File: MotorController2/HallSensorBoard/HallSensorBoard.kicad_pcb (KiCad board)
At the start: 2 copper layers, 13 x 23 mm, 6 parts, among them J1 Conn_01x07, J2 Conn_01x02, U1 S49E, U2 S49E, U3 S49E

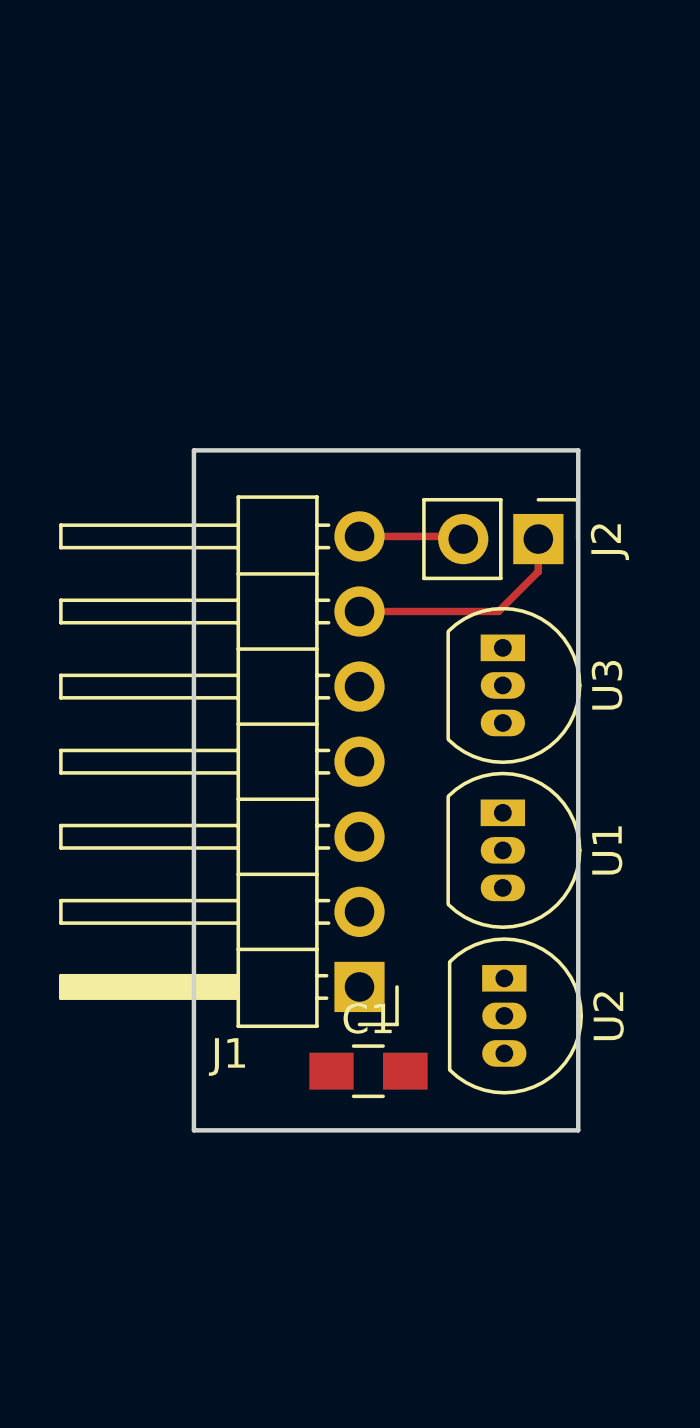
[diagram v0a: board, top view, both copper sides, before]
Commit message: Final board.
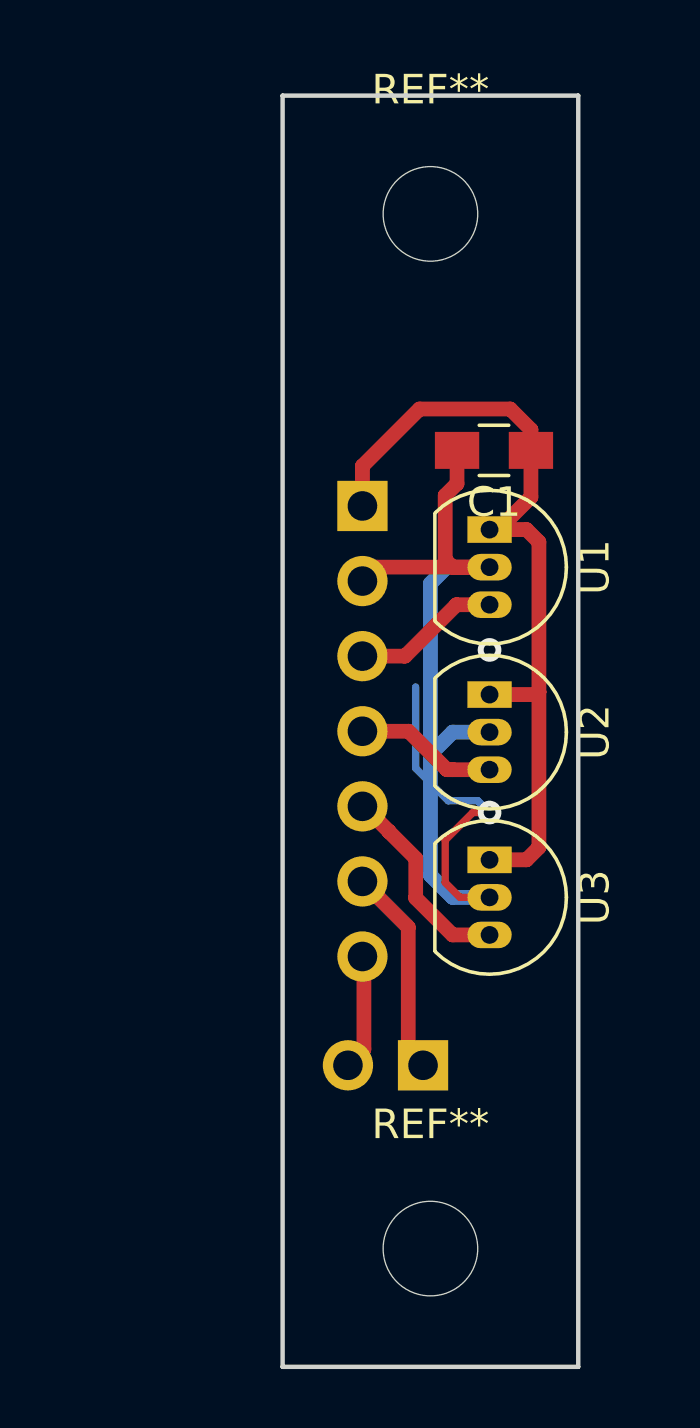
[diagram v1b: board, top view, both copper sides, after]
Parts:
- added REF**: MountingHole_3.2mm_M3, Mounting_Holes:MountingHole_3.2mm_M3, F.Cu at (156.0, 90.0)
- added REF**: MountingHole_3.2mm_M3, Mounting_Holes:MountingHole_3.2mm_M3, F.Cu at (156.0, 125.0)
- J1, J2: moved to B.Cu
- moved C1 21.4 mm to (158.2, 98.0), turned to 180 degrees
- moved J2 18.2 mm to (155.8, 118.8), turned to 90 degrees
- moved J1 16.3 mm to (153.7, 99.9)
- moved U2 9.61 mm to (158.0, 106.3)
- moved U1 4.03 mm to (158.0, 100.7)
- moved U3 1.65 mm to (158.0, 111.8)
- renumbered U3 to U1, U1 to U3
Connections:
- U1 pad 3: Net-(J1-Pad5) -> Net-(J1-Pad3)
- U3 pad 3: Net-(J1-Pad3) -> Net-(J1-Pad5)
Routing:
- net GND: track 0.00 -> 37.6 mm, vias 0 -> 2
- net +3V3: track 0.00 -> 28.0 mm
- net Net-(J1-Pad5): track 0.00 -> 6.84 mm
- net Net-(J1-Pad3): track 0.00 -> 4.97 mm
- net Net-(J1-Pad4): track 0.00 -> 4.79 mm
- net Net-(J1-Pad6): track 7.71 -> 9.19 mm
- added copper zone on B.Cu, net GND
- added copper zone on F.Cu, net GND
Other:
- board size 13 x 23 mm -> 10 x 43 mm
